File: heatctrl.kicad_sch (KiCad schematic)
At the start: 2 parts, among them J1 Conn_01x10_Pin, U1 T-Display-S3

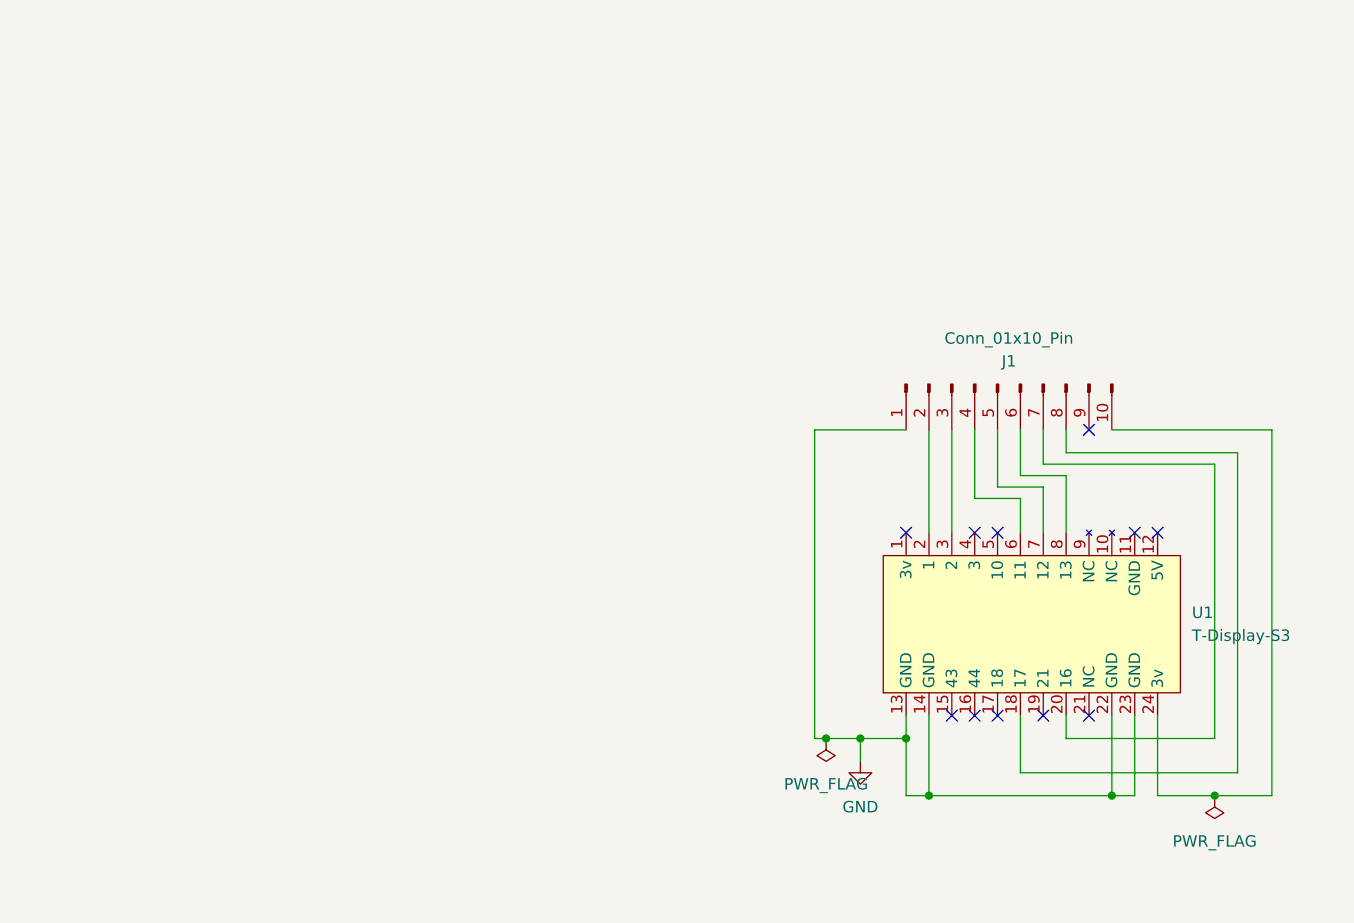
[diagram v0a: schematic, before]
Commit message: mcp and t-display-s3
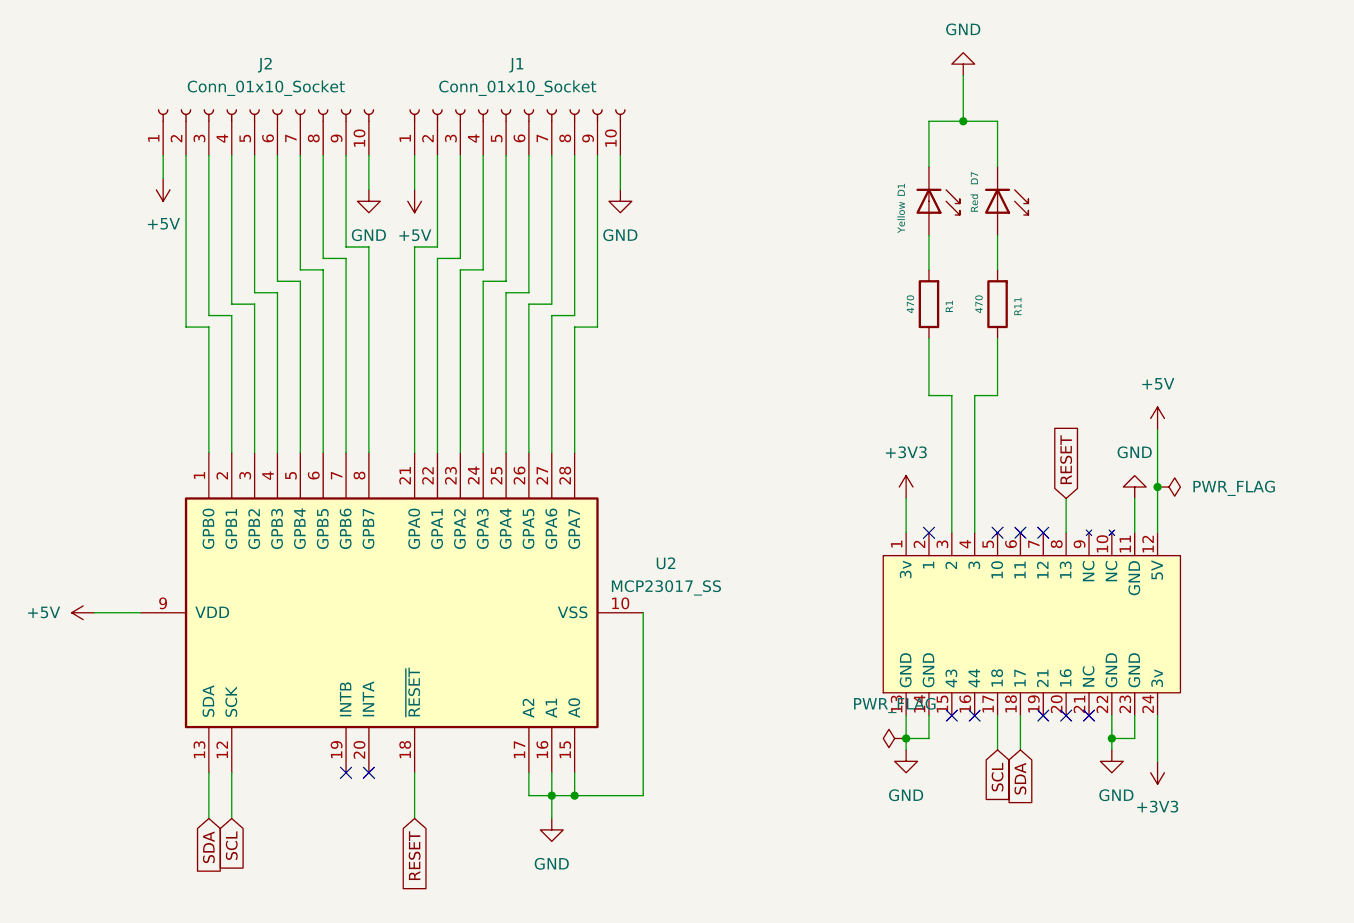
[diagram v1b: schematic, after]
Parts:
- removed J1: Conn_01x10_Pin, Connector_PinSocket_2.54mm:PinSocket_1x10_P2.54mm_Vertical, symbol Connector:Conn_01x10_Pin
- added D1: Yellow, PCM_JLCPCB:D_0805, symbol PCM_JLCPCB-Diodes:LED,0805,Yellow
- added D7: Red, PCM_JLCPCB:D_0805, symbol PCM_JLCPCB-Diodes:LED,0805,Red
- added J1, J2: Conn_01x10_Socket, Connector_PinSocket_2.54mm:PinSocket_1x10_P2.54mm_Vertical, symbol Connector:Conn_01x10_Socket
- added R1, R11: 470, Resistor_SMD:R_0603_1608Metric, symbol Device:R
- added U2: MCP23017_SS, Package_SO:SSOP-28_5.3x10.2mm_P0.65mm, symbol HV_SYM01:MCP23017_SS
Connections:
- net GND: now also U1.11 (GND), D1.1, D7.1, J1.10 (Pin_10), J2.10 (Pin_10), U2.10 (VSS), U2.15 (A0), U2.16 (A1), U2.17 (A2)
- net +3V3: now reaches U1.1 (3v)
- net +3V3: now also U1.24 (3v)
- net +5V: now reaches U1.12 (5V)
- net +5V: now also J1.1 (Pin_1), J2.1 (Pin_1), U2.9 (VDD)
- net SCL: now reaches U1.17 (18)
- net SCL: now also U2.12 (SCK)
- net SDA: now reaches U1.18 (17)
- net SDA: now also U2.13 (SDA)
- net at U1.3 (2): now also R1.1
- net at U1.4 (3): now also R11.1
- net RESET: now reaches U1.8 (13)
- net RESET: now also U2.18 (~{RESET})
- new net: D7.2, R11.2
- new net: D1.2, R1.2
- new net: J1.2 (Pin_2), U2.21 (GPA0)
- new net: J1.3 (Pin_3), U2.22 (GPA1)
- new net: J1.4 (Pin_4), U2.23 (GPA2)
- new net: J1.5 (Pin_5), U2.24 (GPA3)
- new net: J1.6 (Pin_6), U2.25 (GPA4)
- new net: J1.7 (Pin_7), U2.26 (GPA5)
- new net: J1.8 (Pin_8), U2.27 (GPA6)
- new net: J1.9 (Pin_9), U2.28 (GPA7)
- new net: J2.2 (Pin_2), U2.1 (GPB0)
- new net: J2.3 (Pin_3), U2.2 (GPB1)
- new net: J2.4 (Pin_4), U2.3 (GPB2)
- new net: J2.5 (Pin_5), U2.4 (GPB3)
- new net: J2.6 (Pin_6), U2.5 (GPB4)
- new net: J2.7 (Pin_7), U2.6 (GPB5)
- new net: J2.8 (Pin_8), U2.7 (GPB6)
- new net: J2.9 (Pin_9), U2.8 (GPB7)
